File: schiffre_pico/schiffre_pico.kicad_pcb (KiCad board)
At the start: 2 copper layers, 70 x 50 mm, 6 parts, among them U5 Pico

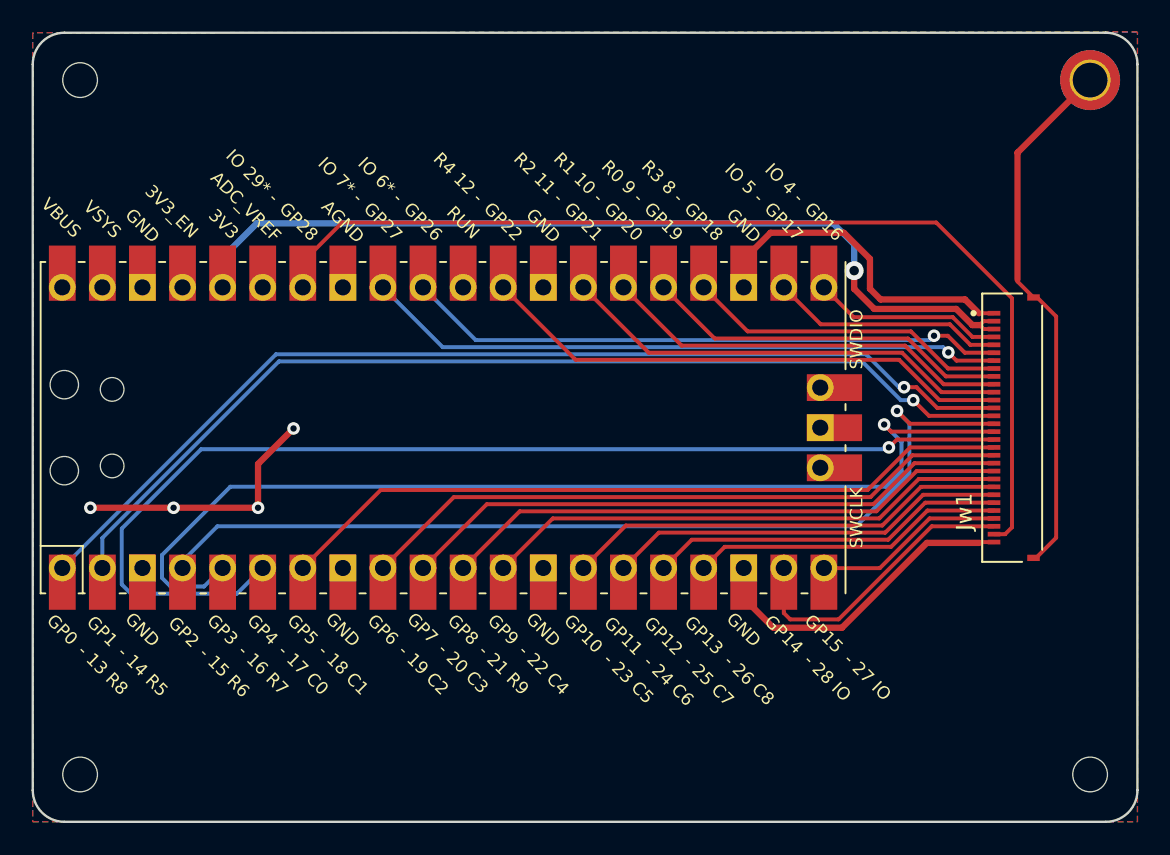
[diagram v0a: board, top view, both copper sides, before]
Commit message: small drc things
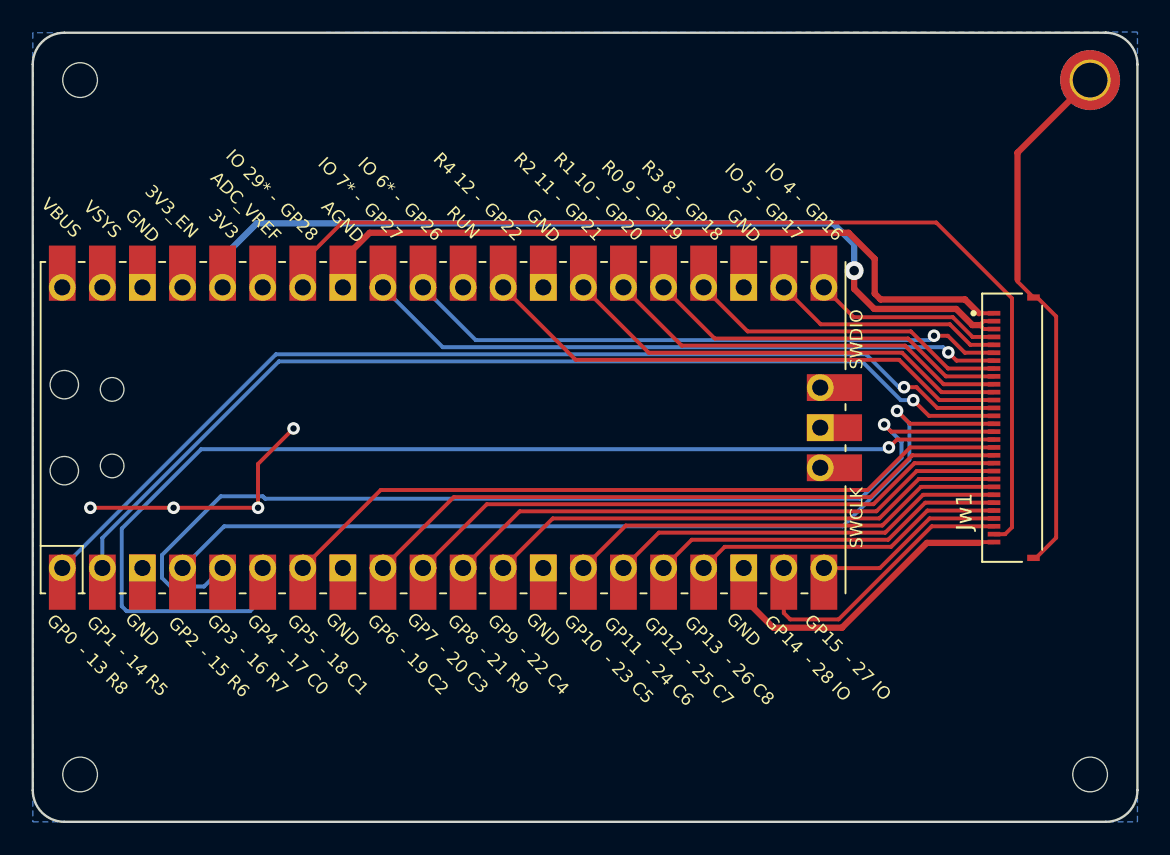
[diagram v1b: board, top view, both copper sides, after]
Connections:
- U5 pad 13: unconnected-(U5-GND-Pad13) -> GND
- U5 pad 35: GND -> unconnected-(U5-ADC_VREF-Pad35)
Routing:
- net GND: track 58.9 -> 84.5 mm
- net /GPIO4: track 71.0 -> 73.9 mm
- net /GPIO2: track 59.5 -> 58.8 mm
- removed copper zone on F.Cu, net GND
